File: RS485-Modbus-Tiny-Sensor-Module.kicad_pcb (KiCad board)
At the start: 2 copper layers, 49.5 x 47 mm, 23 parts, among them SW1 FSM4JSMA, U2 ATtiny3216-S

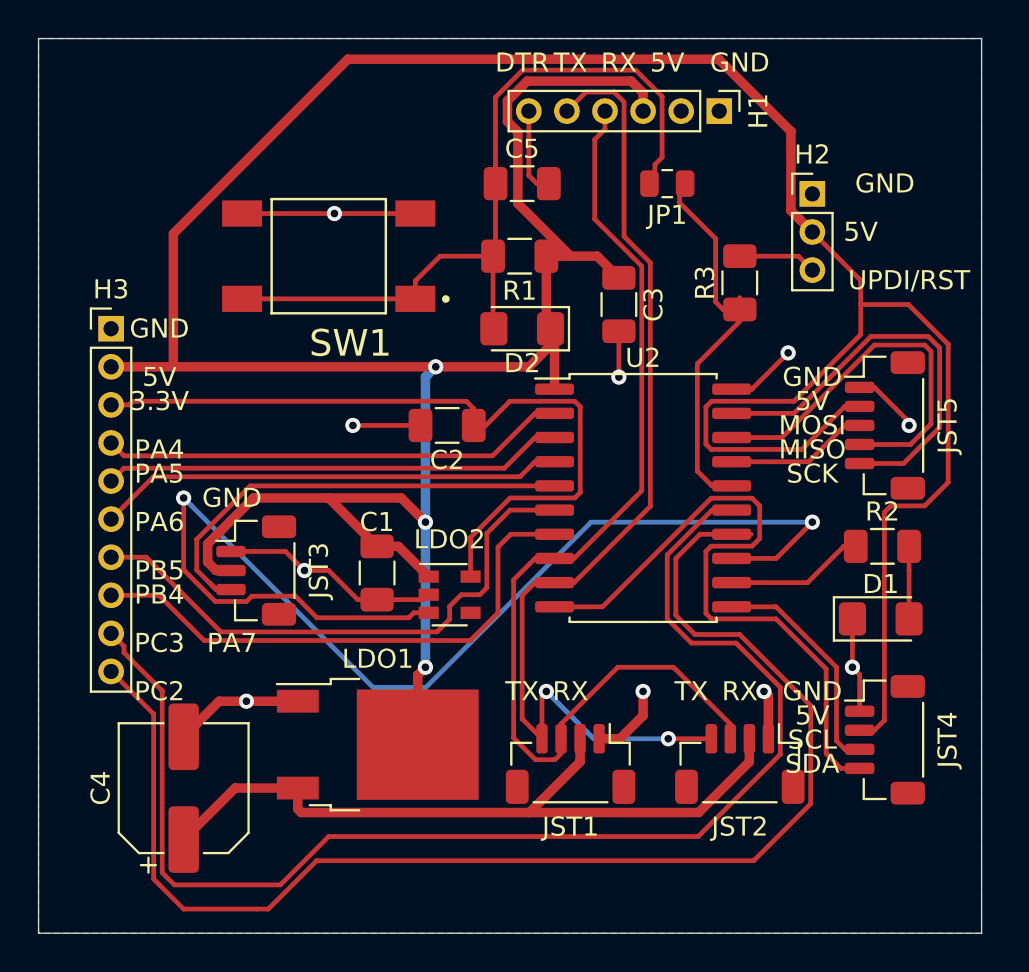
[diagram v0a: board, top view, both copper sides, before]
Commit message: Add files via upload
PCB V1.0
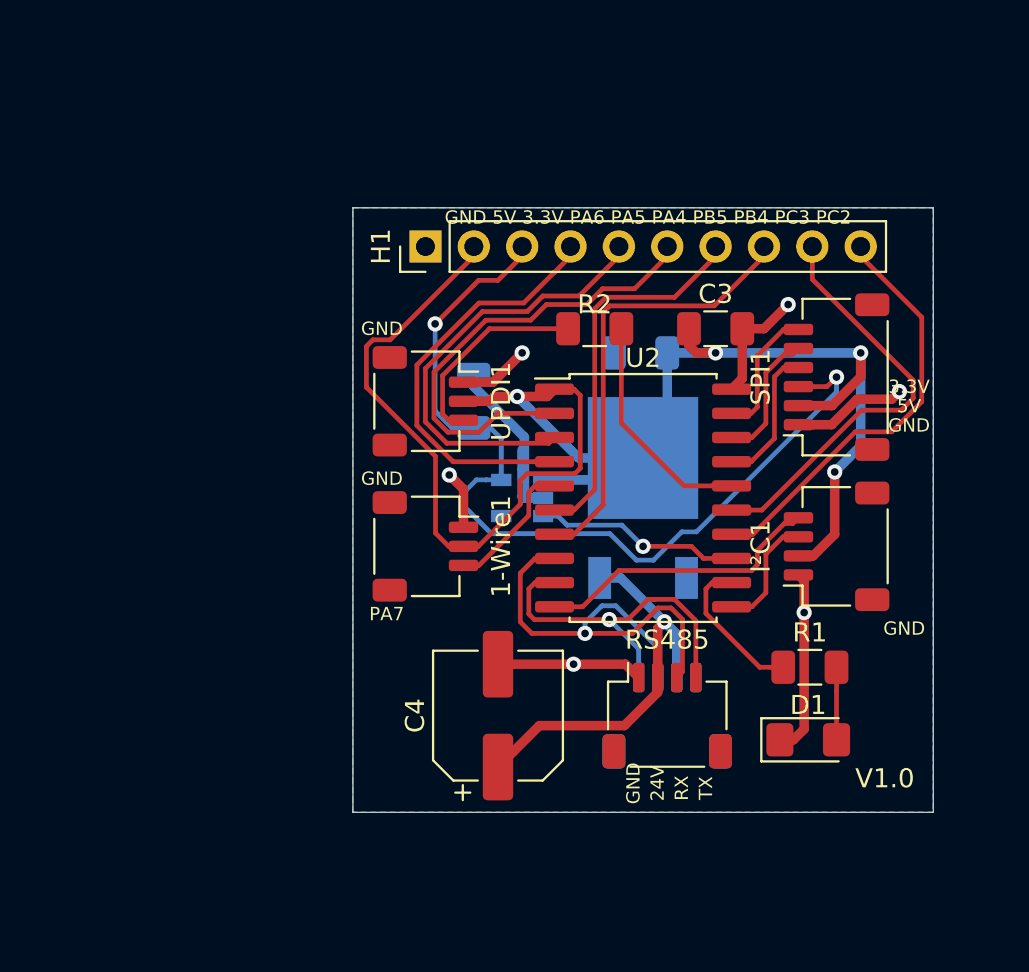
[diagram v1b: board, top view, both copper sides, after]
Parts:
- removed C5: 1u, Capacitor_SMD:C_1206_3216Metric
- removed D2: D, Diode_SMD:D_1206_3216Metric_Pad1.42x1.75mm_HandSolder
- removed H2: Conn_01x03, Connector_PinHeader_2.00mm:PinHeader_1x03_P2.00mm_Vertical
- removed H3: Conn_01x10, Connector_PinHeader_2.00mm:PinHeader_1x10_P2.00mm_Vertical
- removed JP1: Jumper, Resistor_SMD:R_0805_2012Metric
- removed the R1 at (191.6, 86.4)
- removed SW1: FSM4JSMA, FSM4JSMA:TE_FSM4JSMA
- added UPDI1: Conn_01x03, Connector_JST:JST_SH_SM03B-SRSS-TB_1x03-1MP_P1.00mm_Horizontal, F.Cu at (186.7, 94.0)
- 1-Wire1: renamed from JST3; footprint Connector_JST:JST_SH_BM03B-SRSS-TB_1x03-1MP_P1.00mm_Vertical -> Connector_JST:JST_SH_SM03B-SRSS-TB_1x03-1MP_P1.00mm_Horizontal
- C1, C2, LDO1, LDO2: moved to B.Cu
- H1: value Conn_01x06 -> Conn_01x10; footprint Connector_PinHeader_2.00mm:PinHeader_1x06_P2.00mm_Vertical -> Connector_PinHeader_2.54mm:PinHeader_1x10_P2.54mm_Vertical
- I²C1: renamed from JST4; footprint Connector_JST:JST_SH_BM04B-SRSS-TB_1x04-1MP_P1.00mm_Vertical -> Connector_JST:JST_SH_SM04B-SRSS-TB_1x04-1MP_P1.00mm_Horizontal
- RS485: renamed from JST1; footprint Connector_JST:JST_SH_BM04B-SRSS-TB_1x04-1MP_P1.00mm_Vertical -> Connector_JST:JST_SH_SM04B-SRSS-TB_1x04-1MP_P1.00mm_Horizontal
- RS485_2: renamed from JST2; footprint Connector_JST:JST_SH_BM04B-SRSS-TB_1x04-1MP_P1.00mm_Vertical -> Connector_JST:JST_SH_SM04B-SRSS-TB_1x04-1MP_P1.00mm_Horizontal; moved to B.Cu
- SPI1: renamed from JST5; value Conn_01x05 -> Conn_01x06; footprint Connector_JST:JST_SH_BM05B-SRSS-TB_1x05-1MP_P1.00mm_Vertical -> Connector_JST:JST_SH_SM06B-SRSS-TB_1x06-1MP_P1.00mm_Horizontal
- moved LDO1 19.0 mm to (198.1, 99.1), turned to 90 degrees
- moved C1 18.0 mm to (198.0, 91.4), turned to 180 degrees
- moved H1 17.0 mm to (186.7, 85.9), turned to 90 degrees
- moved C4 16.9 mm to (190.5, 110.5)
- moved I²C1 10.5 mm to (208.3, 101.6), turned to 90 degrees
- moved 1-Wire1 8.98 mm to (186.7, 101.6)
- moved R2 7.99 mm to (195.6, 90.2), turned to 180 degrees
- moved D1 7.41 mm to (206.8, 111.8)
- moved R1 7.41 mm to (206.9, 108.0)
- moved LDO2 6.35 mm to (191.8, 99.1), turned to 180 degrees
- moved RS485 5.68 mm to (199.4, 110.5), turned to 0 degrees
- moved C3 5.24 mm to (201.9, 90.2), turned to 0 degrees
- moved RS485_2 4.58 mm to (199.4, 110.5)
- moved SPI1 3.59 mm to (208.3, 92.7), turned to 90 degrees
- moved C2 1.89 mm to (189.2, 94.0), turned to 90 degrees
- renumbered R2 to R1, R3 to R2
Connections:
- H1 pad 2: Net-(H1-Pad2) -> /5V
- H1 pad 3: /5V -> /3.3V
- H1 pad 4: /RX -> /PA6
- H1 pad 5: /TX -> /PA5
- H1 pad 6: /DTR -> /PA4
- R2 pad 2: /UPDI -> Net-(R2-Pad2)
- SPI1 pad 3: /MOSI -> /3.3V
- SPI1 pad 4: /MISO -> /MOSI
- SPI1 pad 5: /SCK -> /MISO
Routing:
- net /5V: track 203.6 -> 88.9 mm, vias 3 -> 4
- net Net-(LDO2-Pad3): track 63.8 -> 10.8 mm, vias 2 -> 1
- net /PC2: track 71.0 -> 21.8 mm
- net /PC3: track 67.9 -> 22.6 mm
- net Net-(C5-Pad1): track 42.7 -> 0.00 mm
- net /TX: track 55.1 -> 19.3 mm, vias 2 -> 1
- net /RX: track 54.9 -> 24.7 mm, vias 0 -> 1
- net /SDA: track 35.4 -> 15.2 mm
- net /24V: track 39.3 -> 21.6 mm, vias 0 -> 1
- net /PA7: track 24.3 -> 7.23 mm
- net /SCK: track 22.0 -> 6.91 mm
- net /MISO: track 20.6 -> 7.01 mm
- net Net-(R2-Pad2): track 0.00 -> 10.9 mm
- net /PB5: track 29.6 -> 19.5 mm
- net /3.3V: track 39.7 -> 47.2 mm, vias 0 -> 2
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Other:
- board size 49.5 x 47 mm -> 30.5 x 31.8 mm
- board text added: "24V"
- board text added: "GND 5V 3.3V PA6 PA5 PA4 PB5 PB4 PC3 PC2"
- board text added: "V1.0"
- board text removed: "DTR"
- board text removed: "MISO"
- board text removed: "MOSI"
- board text removed: "PA4"
- board text removed: "PA5"
- board text removed: "PA6"
- board text removed: "PB4"
- board text removed: "PB5"
- board text removed: "PC2"
- board text removed: "PC3"
- board text removed: "SCK"
- board text removed: "SCL"
- board text removed: "SDA"
- board text removed: "UPDI/RST"
